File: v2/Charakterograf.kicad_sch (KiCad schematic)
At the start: 0 parts

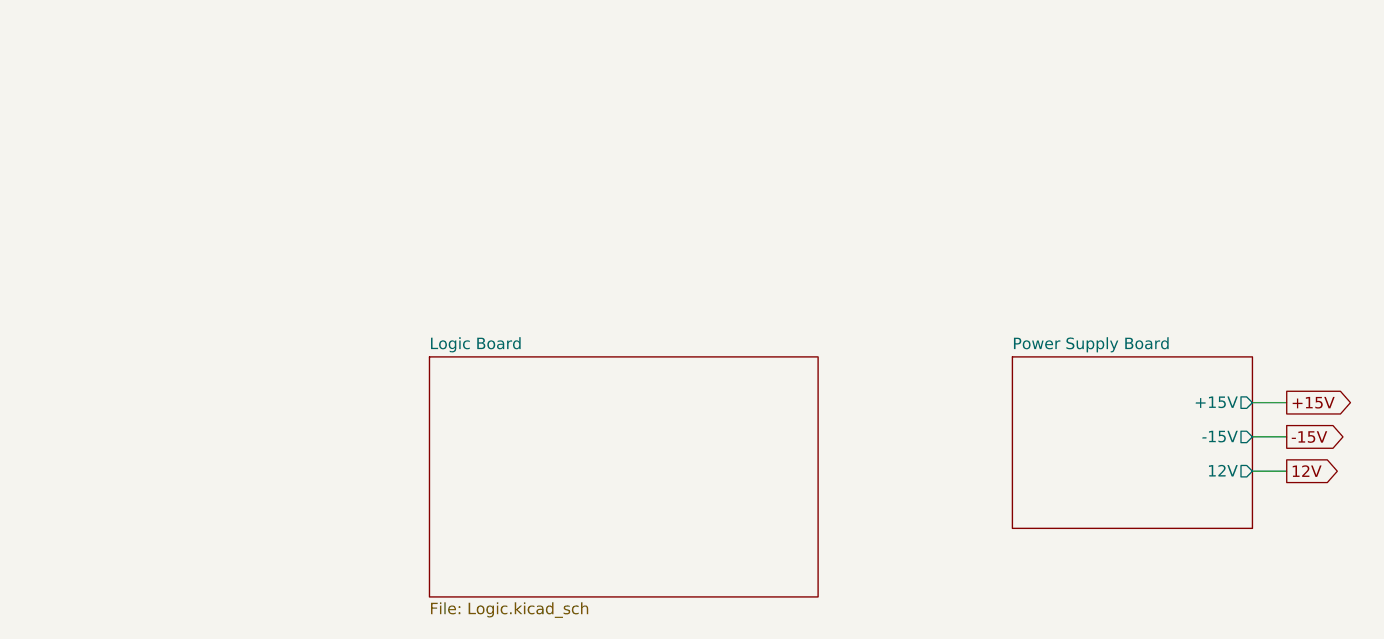
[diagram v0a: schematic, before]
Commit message: Almost finished v2
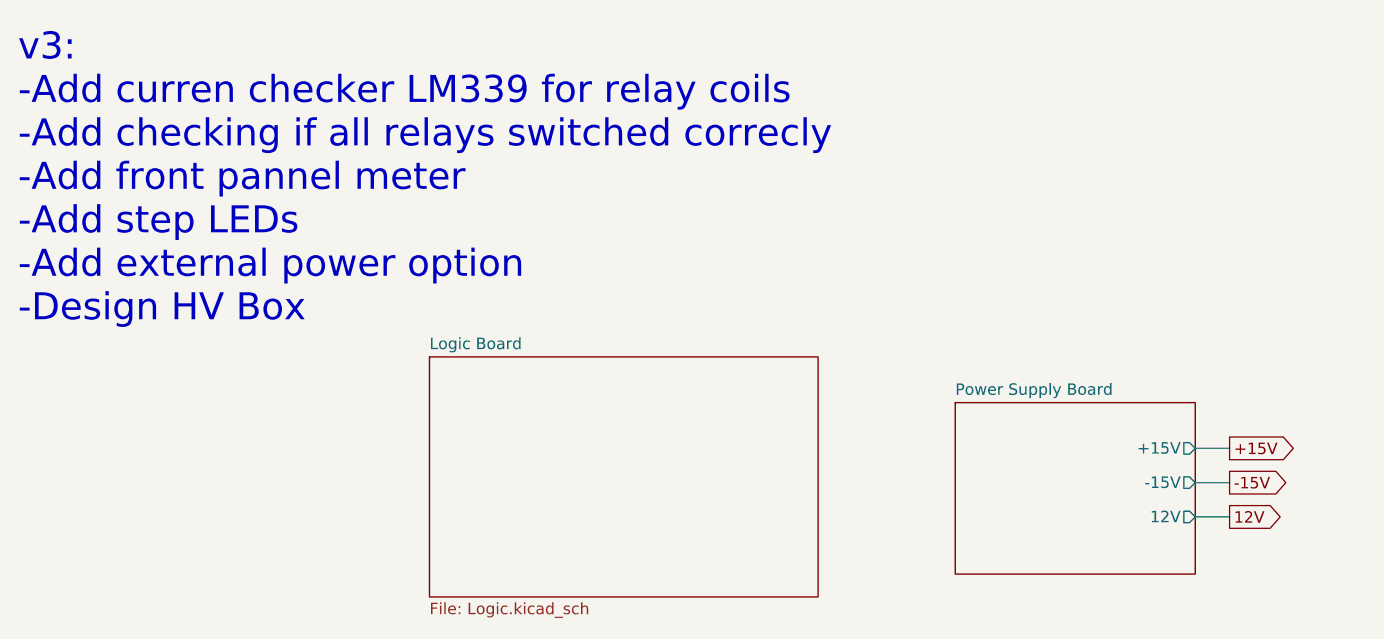
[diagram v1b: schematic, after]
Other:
- note added: "v3: -Add curren checker LM339 for relay coils -Add checking if all relays switched correcly -Add front pannel meter -Add step LEDs -Add external power option -Design HV Box"
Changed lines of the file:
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@@
 		(rev "2")
+	)
+	(text "v3:\n-Add curren checker LM339 for relay coils\n-Add checking if all relays switched correcly\n-Add front pannel meter\n-Add step LEDs\n-Add external power option\n-Design HV Box"
+		(exclude_from_sim no)
+		(at 13.97 29.718 0)
+		(effects
+			(font
+				(size 3 3)
+			)
+			(justify left)
+		)
 	)
 	(wire
 		(pts
-			(xy 154.94 58.42) (xy 151.13 58.42)
+			(xy 148.59 63.5) (xy 144.78 63.5)
 		)
 		(stroke
@@
 	(wire
 		(pts
-			(xy 151.13 54.61) (xy 154.94 54.61)
+			(xy 144.78 59.69) (xy 148.59 59.69)
 		)
 		(stroke
@@
 	(wire
 		(pts
-			(xy 151.13 62.23) (xy 154.94 62.23)
+			(xy 144.78 67.31) (xy 148.59 67.31)
 		)
 		(stroke
@@
 	(global_label "12V"
 		(shape output)
-		(at 154.94 62.23 0)
+		(at 148.59 67.31 0)
 		(fields_autoplaced yes)
 		(effects
@@
 		)
 		(property "Intersheetrefs" "${INTERSHEET_REFS}"
-			(at 161.4328 62.23 0)
+			(at 155.0828 67.31 0)
 			(hide yes)
 			(show_name no)
@@
 	(global_label "+15V"
 		(shape output)
-		(at 154.94 54.61 0)
+		(at 148.59 59.69 0)
 		(fields_autoplaced yes)
 		(effects
@@
 		)
 		(property "Intersheetrefs" "${INTERSHEET_REFS}"
-			(at 163.0052 54.61 0)
+			(at 156.6552 59.69 0)
 			(hide yes)
 			(show_name no)
@@
 	(global_label "-15V"
 		(shape output)
-		(at 154.94 58.42 0)
+		(at 148.59 63.5 0)
 		(fields_autoplaced yes)
 		(effects
@@
 		)
 		(property "Intersheetrefs" "${INTERSHEET_REFS}"
-			(at 163.0052 58.42 0)
+			(at 156.6552 63.5 0)
 			(hide yes)
 			(show_name no)
@@
 	)
 	(sheet
-		(at 124.46 49.53)
+		(at 118.11 54.61)
 		(size 26.67 19.05)
 		(exclude_from_sim no)
@@
 		)
 		(property "Sheetname" "Power Supply Board"
-			(at 124.46 48.8184 0)
+			(at 118.11 53.8984 0)
 			(show_name no)
 			(do_not_autoplace no)
@@
 		)
 		(property "Sheetfile" "power_supply.kicad_sch"
-			(at 124.46 69.1646 0)
+			(at 118.11 74.2446 0)
 			(hide yes)
 			(show_name no)
@@
 		)
 		(pin "+15V" output
-			(at 151.13 54.61 0)
+			(at 144.78 59.69 0)
 			(effects
 				(font
@@
 		)
 		(pin "-15V" output
-			(at 151.13 58.42 0)
+			(at 144.78 63.5 0)
 			(effects
 				(font
@@
 		)
 		(pin "12V" output
-			(at 151.13 62.23 0)
-			(effects
-				(font
+			(at 144.78 67.31 0)
+			(effects
+				(font
